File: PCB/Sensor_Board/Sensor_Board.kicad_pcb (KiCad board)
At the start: 2 copper layers, 90 x 83 mm, 5 parts, among them J1 Conn_01x08_Socket, J2 Conn_01x06_Socket, J3 Conn_01x04_Socket, J4 Conn_01x07_Socket, J5 Conn_01x09_Socket

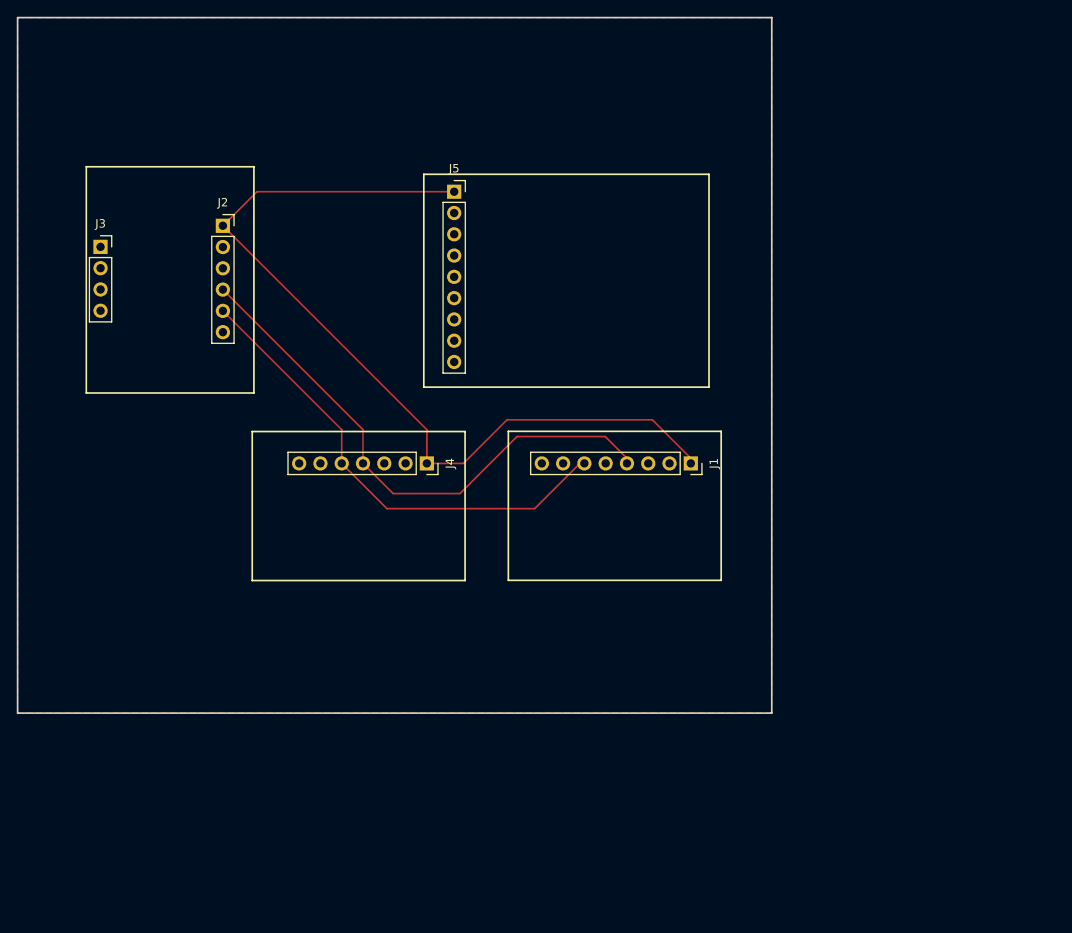
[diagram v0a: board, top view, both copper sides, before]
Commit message: added connector
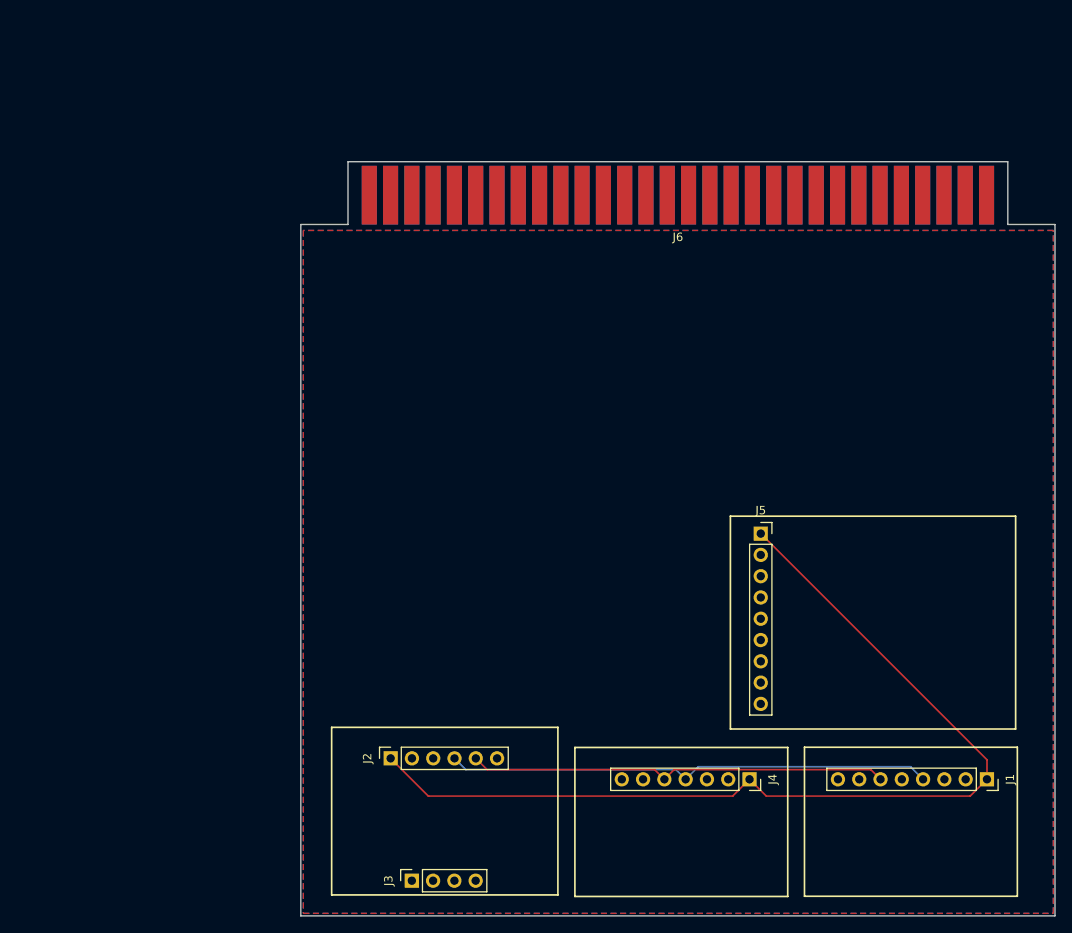
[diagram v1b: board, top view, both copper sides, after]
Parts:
- added J6: SE2-30, SE2-30:SE2-30, F.Cu at (145.2, 63.8)
- moved J3 84.3 mm to (113.4, 145.6), turned to 90 degrees
- moved J2 66.6 mm to (110.9, 131.0), turned to 90 degrees
- moved J5 54.8 mm to (155.1, 104.2)
- moved J4 53.9 mm to (153.7, 133.5)
- moved J1 51.7 mm to (182.1, 133.5)
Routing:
- net +3.3V: track 103.3 -> 116.0 mm
- net /SDA: track 57.8 -> 50.3 mm
- net /SCL: track 64.6 -> 58.2 mm
- added copper zone on B.Cu, net GND
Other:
- board size 90 x 83 mm -> 90 x 90 mm
